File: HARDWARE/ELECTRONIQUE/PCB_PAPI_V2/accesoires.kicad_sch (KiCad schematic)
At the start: 22 parts, among them IC5 ADXL343BCCZ-RL, IC6 MAX98357AETE+, IC8 74HCT1G125GW-Q100H

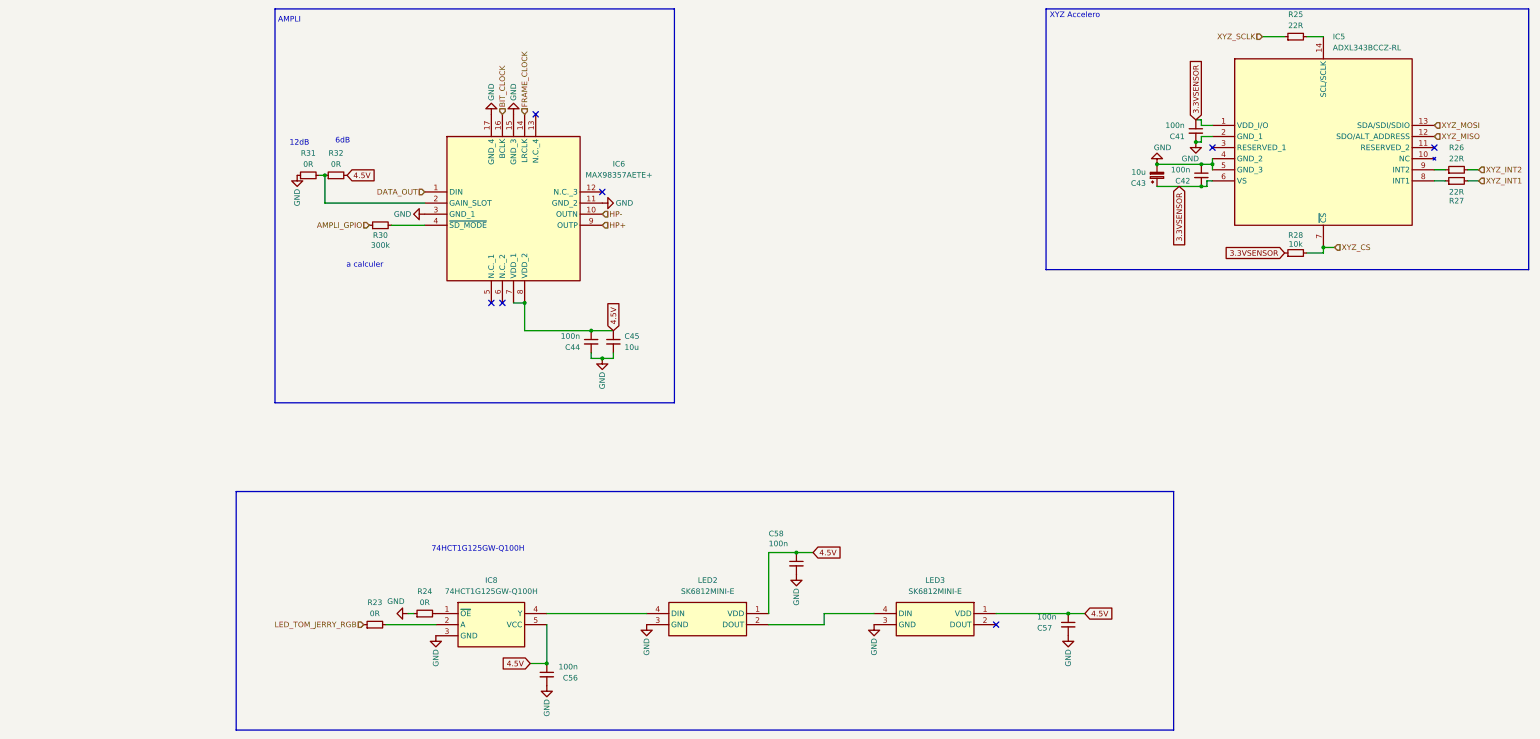
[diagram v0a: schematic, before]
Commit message: up
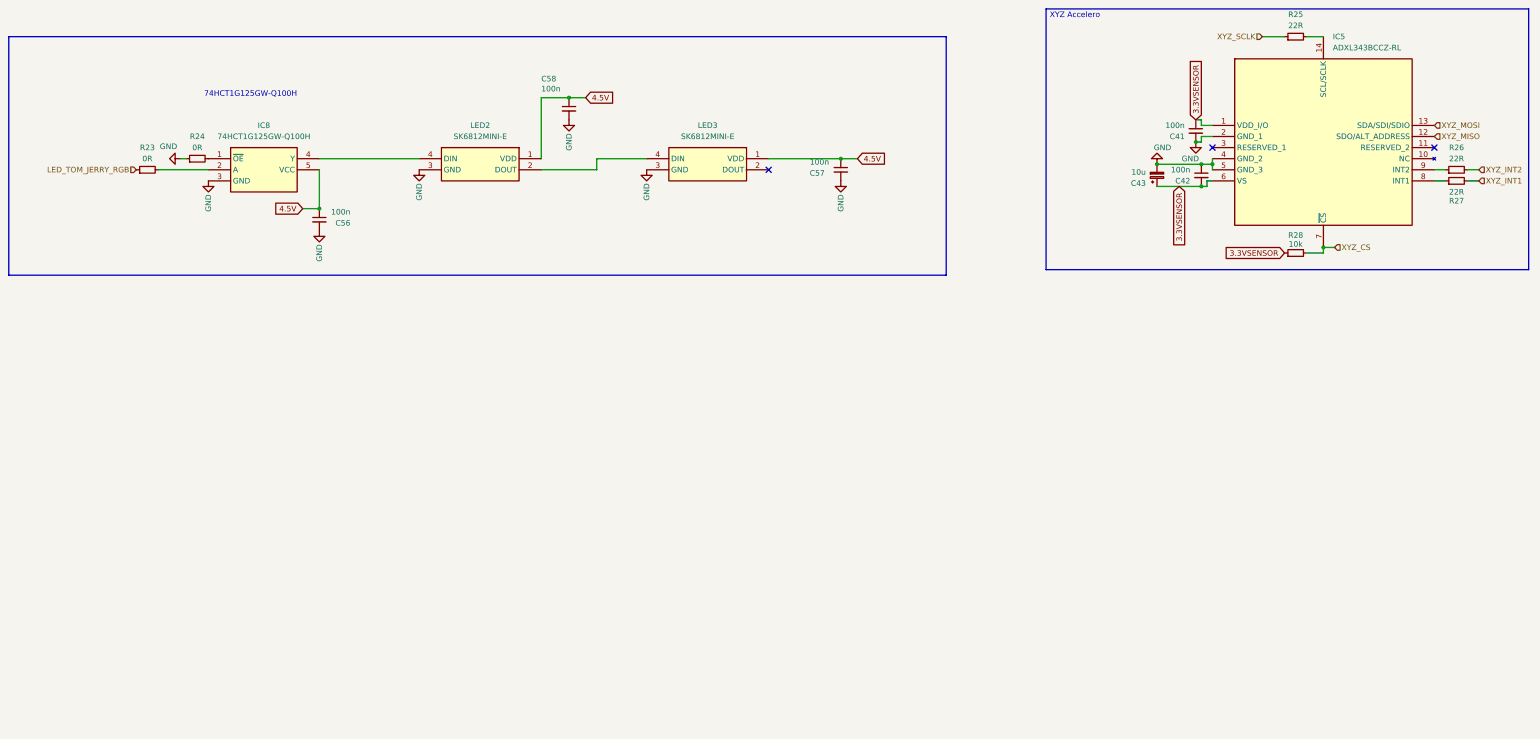
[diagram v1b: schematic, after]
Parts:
- removed C44: 100n, Capacitor_SMD:C_0201_0603Metric, symbol Device:C_Small
- removed C45: 10u, Capacitor_SMD:C_0402_1005Metric, symbol Device:C_Small
- removed IC6: MAX98357AETE+, samacsys:QFN50P300X300X80-17N, symbol samacsys:MAX98357AETE+
- removed R30: 300k, Resistor_SMD:R_0201_0603Metric, symbol Device:R_Small
- removed R31: 0R, samacsys:R_0201_custom, symbol Device:R_Small
- removed R32: 0R, Resistor_SMD:R_0201_0603Metric, symbol Device:R_Small
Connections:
- no-connect marks 7 -> 3
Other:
- note removed: "12dB"
- note removed: "6dB"
- note removed: "AMPLI"
- note removed: "a calculer"
- moved on the sheet: C56, C57, C58, IC8, LED2, LED3, R23, R24
